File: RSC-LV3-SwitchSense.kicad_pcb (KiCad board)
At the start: 2 copper layers, 140 x 85 mm, 171 parts, among them J1 FTSH-105-01-L-DV-K-A, J10 Molex 43045-0400, J11 Molex 43045-0400, J12 Molex 43045-0400, J13 Molex 43045-0400, J14 Molex 43045-0400, J15 Molex 43045-0400, J16 Molex 43650-0200, J2 USB_C_Receptacle_USB2.0_16P, J3 Molex 43650-0500, J4 Molex 43650-0500, J5 Molex 43650-0200, J6 Molex 43045-0400, J7 Molex 43045-0400, J8 Molex 43045-0400, J9 Molex 43045-0400, Q1 AO3400A, Q10 AO3400A, Q2 AO3400A, Q3 AO3400A, Q4 AO3400A, Q5 AO3400A, Q6 AO3400A, Q7 AO3400A, Q8 AO3400A, Q9 AO3400A, U1 STM32G0B1CBTx, U2 TPS54302, U3 TLV74033PDBVR, U4 TJA1051T-3, U5 TJA1051T-3, Y1 Crystal_GND24, Y2 32.768 kHz 6pF

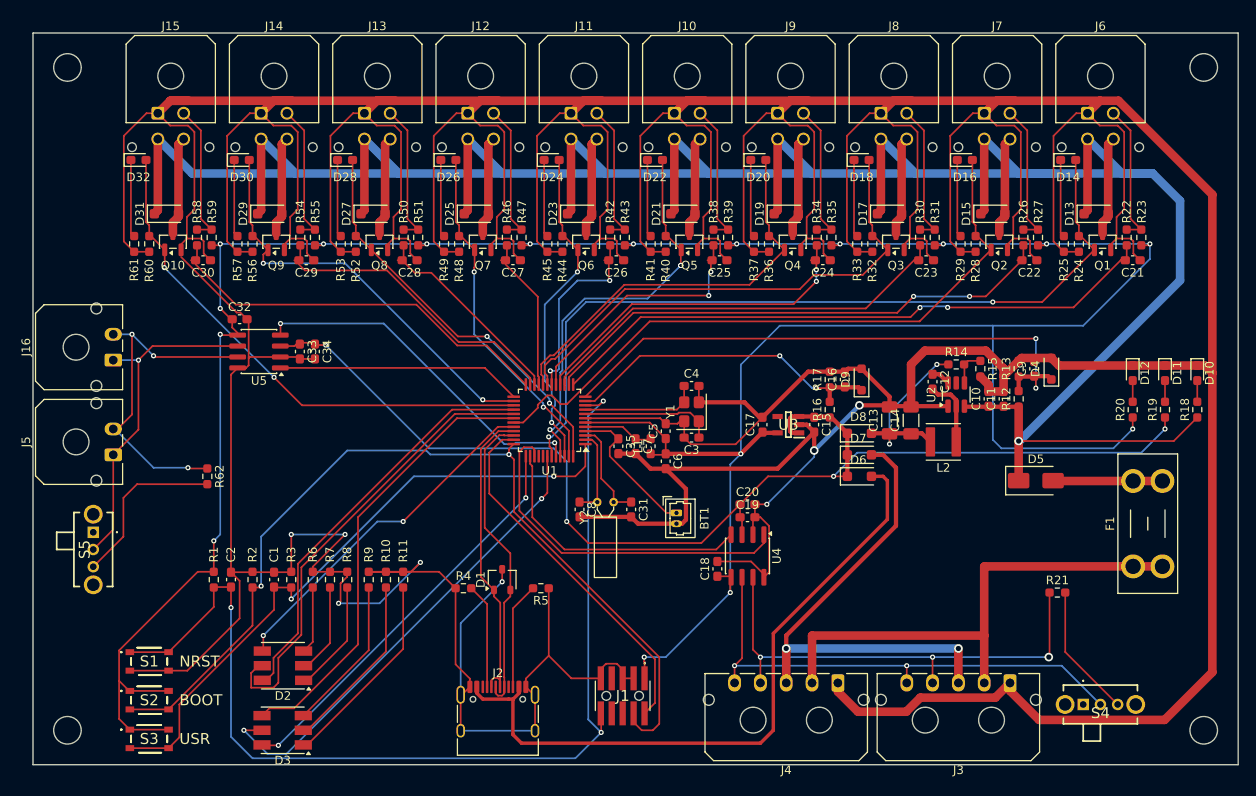
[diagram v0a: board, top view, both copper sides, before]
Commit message: silkscreen work
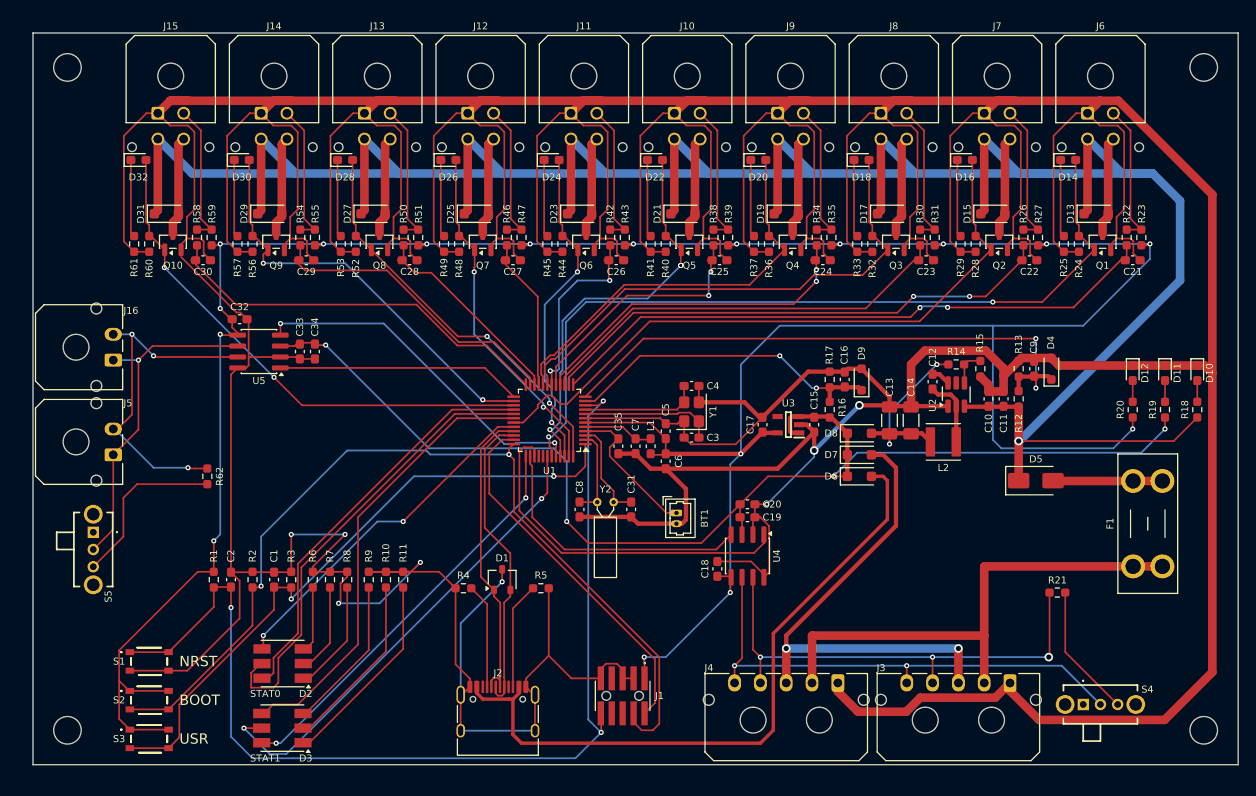
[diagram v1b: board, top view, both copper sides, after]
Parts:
- moved D2 0.25 mm to (99.0, 123.2)
- moved D3 0.25 mm to (99.0, 130.8)
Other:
- board text added: "STAT0"
- board text added: "STAT1"
